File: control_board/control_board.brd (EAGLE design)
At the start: 112.5 x 40 mm, 86 parts, among them X1 VERTICAL_3_5MM_SOCKET

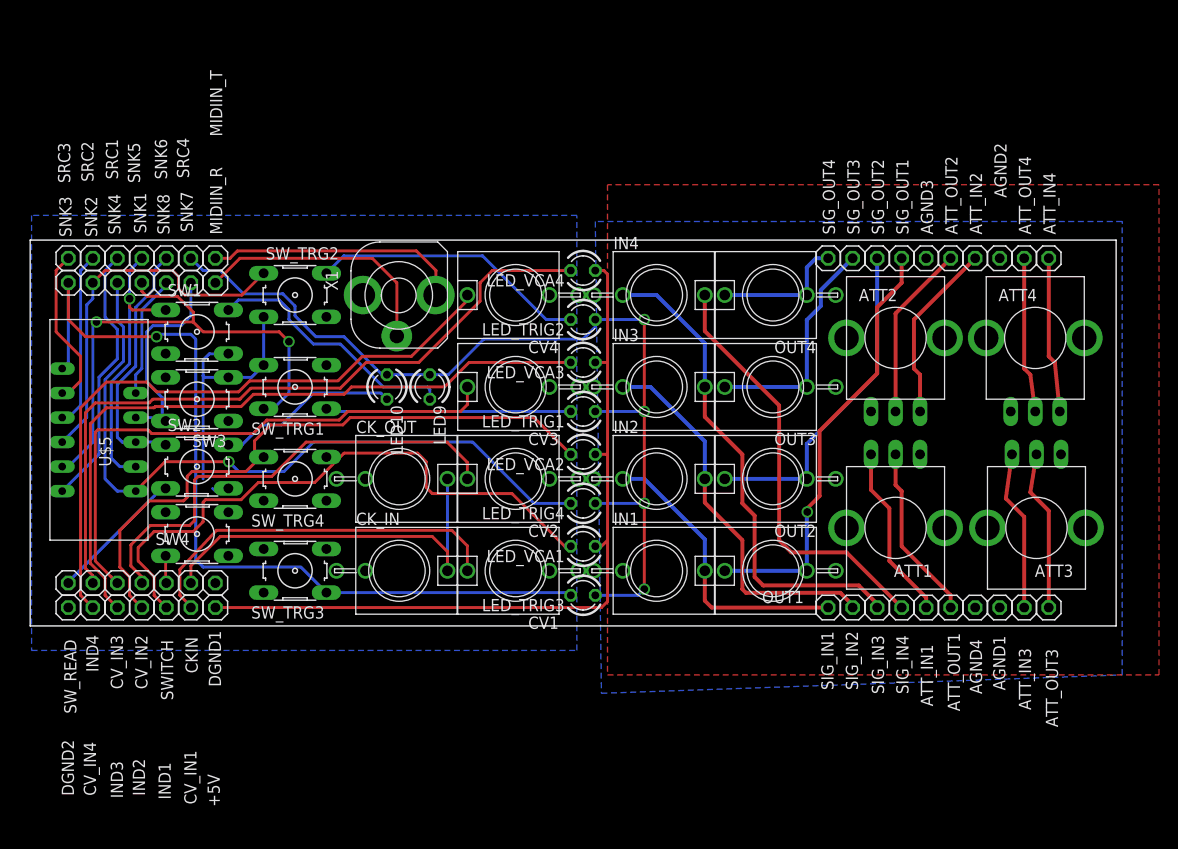
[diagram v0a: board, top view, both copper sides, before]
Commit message: in work
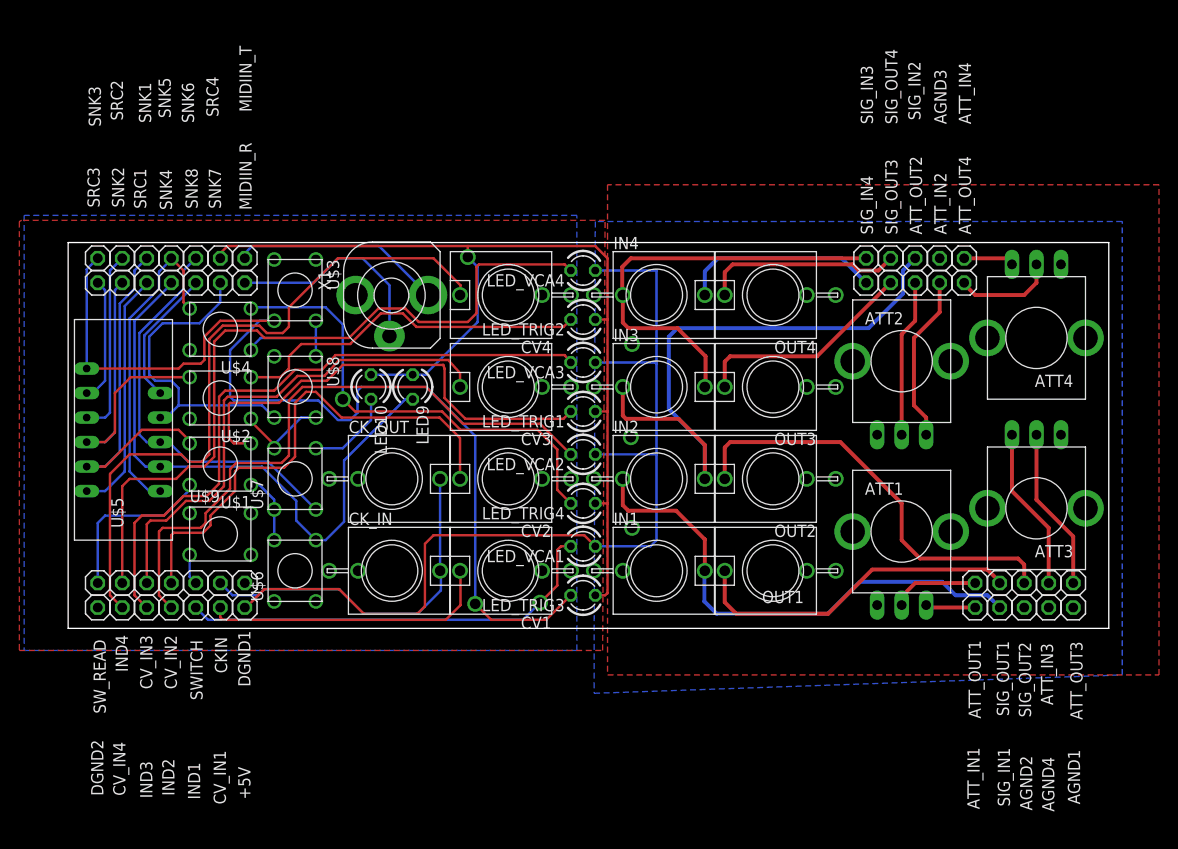
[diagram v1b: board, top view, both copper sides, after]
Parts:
- removed SW1, SW2, SW3, SW4, SW_TRG1, SW_TRG2, SW_TRG3, SW_TRG4: (no value), switch-omron:B3F-10XX
- added U$1, U$2, U$3, U$4, U$6, U$7, U$8, U$9: 6MM_TACT, jason_eagle6:6MMTACT
- moved SIG_OUT2 36.9 mm to (111.8, 38.7)
- moved SIG_IN2 36.8 mm to (100.5, 72.4)
- moved AGND2 36.3 mm to (111.8, 36.2)
- moved SIG_IN3 36.2 mm to (95.4, 72.4)
- moved SIG_OUT1 35.2 mm to (109.2, 38.7)
- moved SIG_IN4 33.9 mm to (95.4, 69.8)
- moved SIG_IN1 17.8 mm to (109.2, 36.2)
- moved ATT_IN4 8.76 mm to (105.5, 72.4)
- moved AGND1 7.62 mm to (116.8, 36.2)
- moved AGND4 7.62 mm to (114.3, 36.2)
- moved ATT_OUT4 6.72 mm to (105.5, 69.8)
- moved SIG_OUT4 6.48 mm to (97.9, 72.4)
- moved SNK4 6.14 mm to (23.4, 72.4)
- moved ATT_IN1 5.08 mm to (106.7, 36.2)
- moved SIG_OUT3 4.69 mm to (97.9, 69.8)
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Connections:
- net GND: now also U$9.1, U$9.4; no longer SW4.3, SW4.4
- net N$18: no longer OUT1.P$2
- net N$26: no longer OUT3.P$2
- net N$27: no longer OUT2.P$2
- net N$28: no longer OUT4.P$2
- net SINK1: now also U$1.2, U$1.3; no longer SW_TRG1.1, SW_TRG1.2
- net SINK2: now also U$2.2, U$2.3; no longer SW_TRG2.1, SW_TRG2.2
- net SINK3: now also U$3.2, U$3.3; no longer SW_TRG3.1, SW_TRG3.2
- net SINK4: now also U$4.2, U$4.3; no longer SW_TRG4.1, SW_TRG4.2
- net SINK5: now also U$6.2, U$6.3; no longer SW1.1, SW1.2
- net SINK6: now also U$7.2, U$7.3; no longer SW2.1, SW2.2
- net SINK7: now also U$8.2, U$8.3; no longer SW3.1, SW3.2
- net SWITCH: now also U$9.2, U$9.3; no longer SW4.1, SW4.2
- net SW_READ: now also U$1.1, U$1.4, U$2.1, U$2.4, U$3.1, U$3.4, U$4.1, U$4.4, U$6.1, U$6.4, U$7.1, U$7.4, U$8.1, U$8.4; no longer SW1.3, SW1.4, SW2.3, SW2.4, SW3.3, SW3.4, SW_TRG1.3, SW_TRG1.4, SW_TRG2.3, SW_TRG2.4, SW_TRG3.3, SW_TRG3.4, SW_TRG4.3, SW_TRG4.4
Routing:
- net N$12: track 44.2 -> 20.8 mm
- net N$10: track 40.1 -> 62.8 mm
- net N$9: track 30.5 -> 52.7 mm
- net N$25: track 80.4 -> 99.5 mm
- net N$21: track 63.1 -> 44.7 mm, vias 0 -> 1
- net SINK3: track 90.5 -> 105.8 mm
- net N$2: track 18.2 -> 5.19 mm
- net N$8: track 16.2 -> 5.22 mm
- net SINK7: track 22.5 -> 33.1 mm
- net N$18: track 45.0 -> 34.8 mm, vias 1 -> 0
- net N$27: track 34.4 -> 43.9 mm
- net N$1: track 18.2 -> 9.09 mm
- net N$13: track 39.2 -> 30.2 mm
- net SINK4: track 75.7 -> 82.7 mm
- net N$28: track 14.0 -> 20.7 mm
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- added copper zone on layer 1, net GND
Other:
- board size 112.5 x 40 mm -> 107.8 x 40 mm

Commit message: moar stuffs
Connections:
- net GND: now also CK_IN.P$2, CV1.P$2, CV2.P$2, CV3.P$2, CV4.P$2
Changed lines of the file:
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@@
 <vertex x="7.874" y="76.327"/>
 </polygon>
+<contactref element="CK_IN" pad="P$2"/>
+<contactref element="CV1" pad="P$2"/>
+<contactref element="CV2" pad="P$2"/>
+<contactref element="CV3" pad="P$2"/>
+<contactref element="CV4" pad="P$2"/>
 </signal>
 <signal name="N$17">
